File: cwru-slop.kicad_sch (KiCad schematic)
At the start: 59 parts, among them J1 USB_C_Receptacle_USB2.0_16P, J2 FTSH-105-01-L-DV-007-K, J3 Conn_01x03_Pin, J4 54-00320, U1 TLV9001IDCK, U10 B3U-1000P, U11 TLV9001IDCK, U12 TLV9001IDCK, U2 AP63205WU, U3 TLV75533PDBV, U4 STM32L433CCTx, U5 TPS2116DRL, U6 FXLS8974CFR3, U7 ESDCAN24-2BLY, U8 MCP2562-E-SN, U9 24lc32at-i/ot, Y1 XRCGB24M000F3M00R0

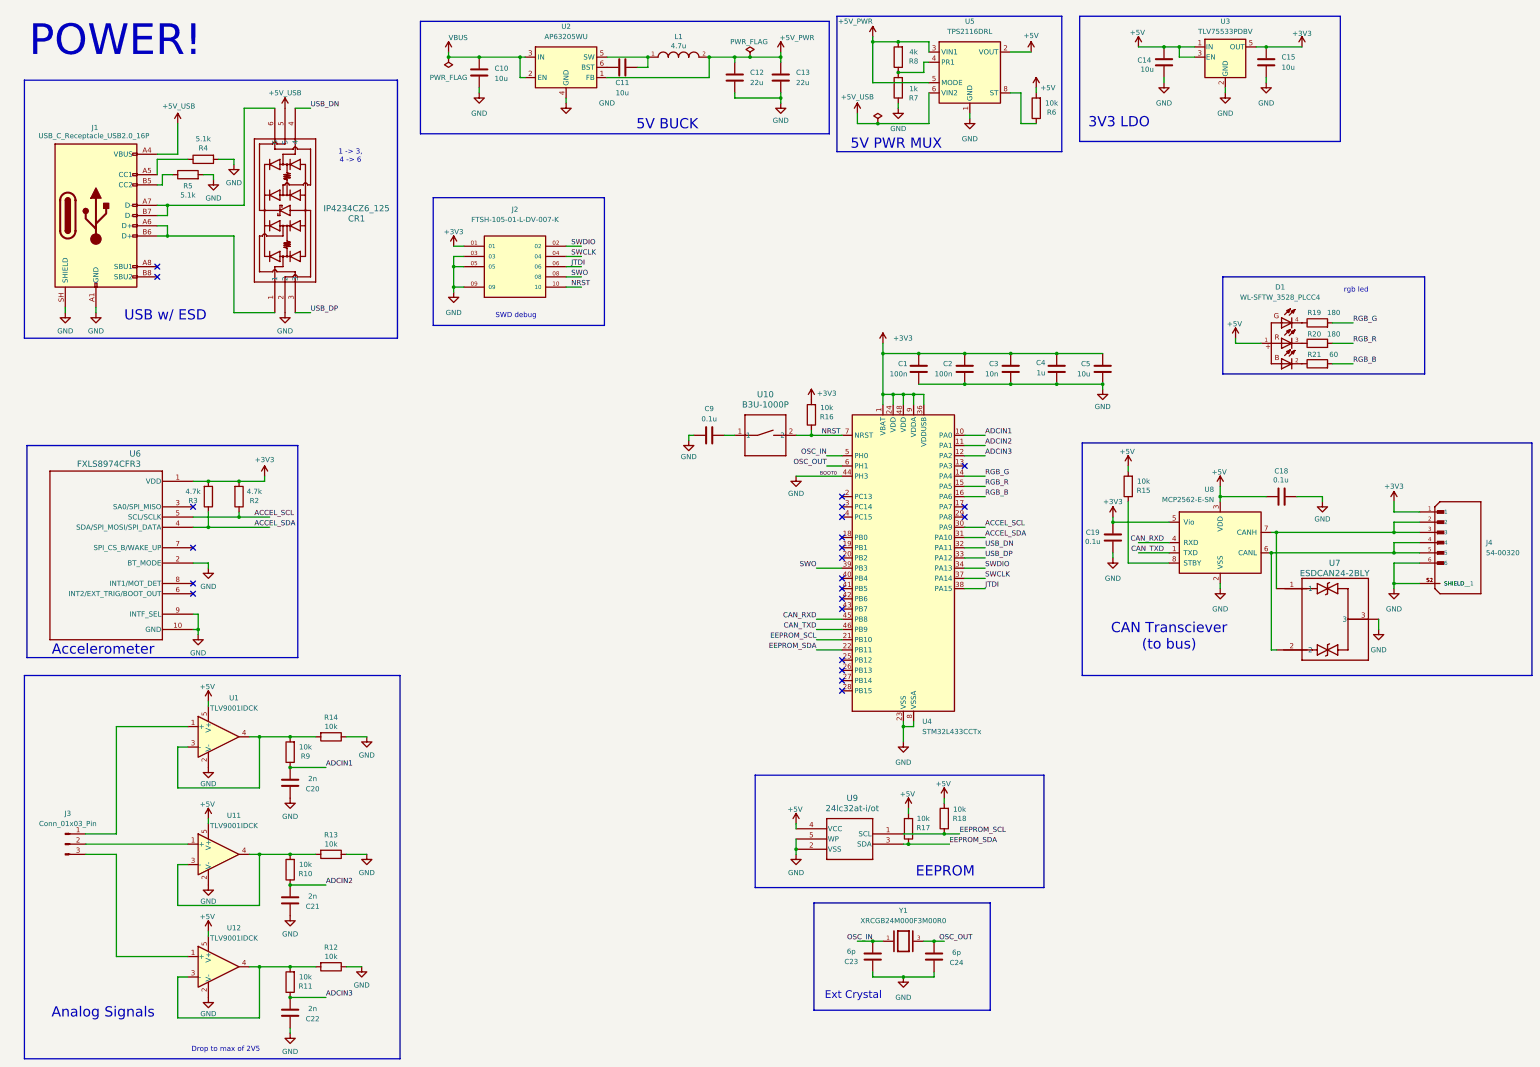
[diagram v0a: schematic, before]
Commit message: led resistor vals
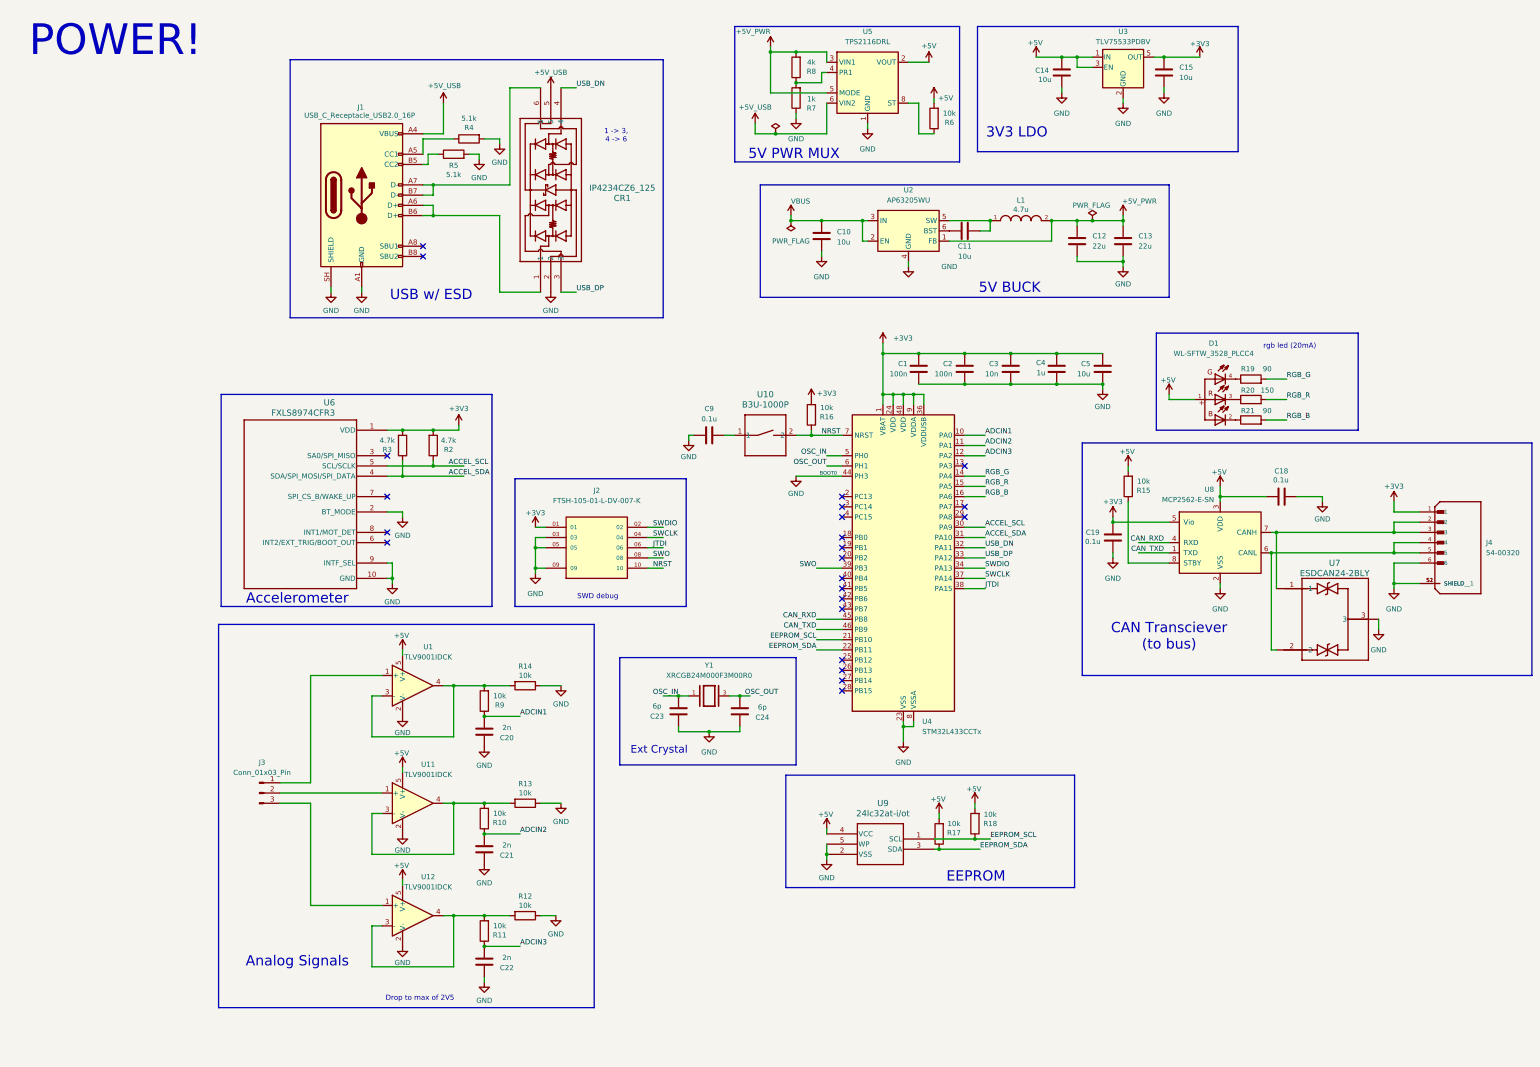
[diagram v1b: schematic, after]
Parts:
- R19: value 180 -> 90
- R20: value 180 -> 150
- R21: value 60 -> 90
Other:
- note added: "rgb led (20mA)"
- note removed: "rgb led"
- moved on the sheet: C10, C11, C12, C13, C14, C15, C20, C21, C22, C23, C24, CR1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
